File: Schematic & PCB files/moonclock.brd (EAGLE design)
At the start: 145 x 38.4 mm, 27 parts, among them U1 TCA9548APWR, U2 ESP32-S2-WROVER-I, U3 AMS1117-3.3, X2 BM04B-SRSS-TB

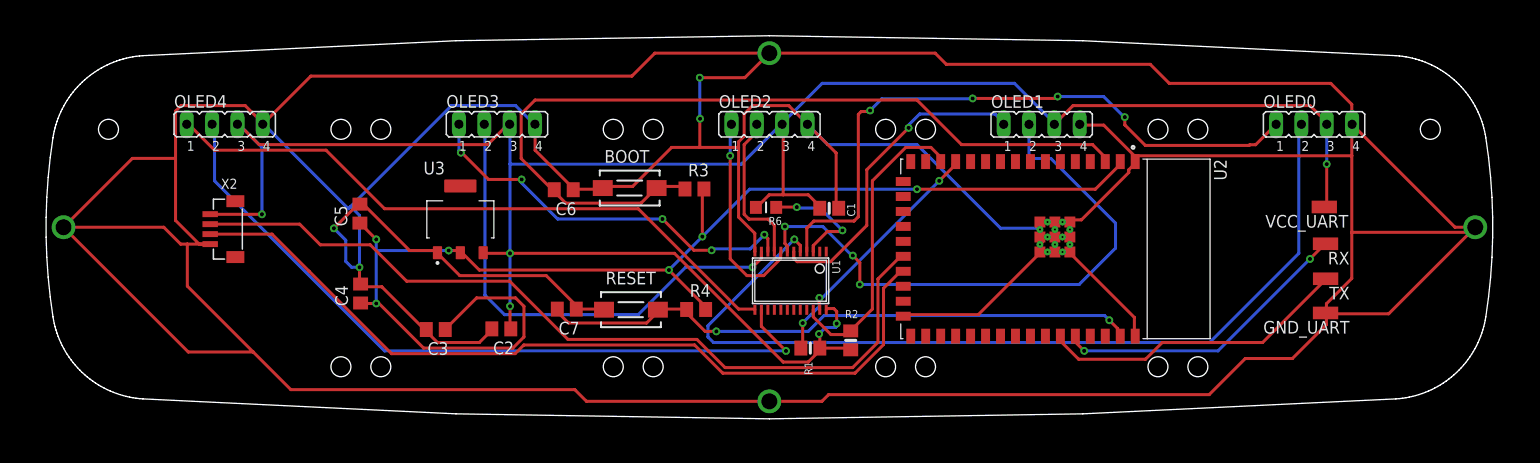
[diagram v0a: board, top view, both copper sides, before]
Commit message: Updated EAGLE files
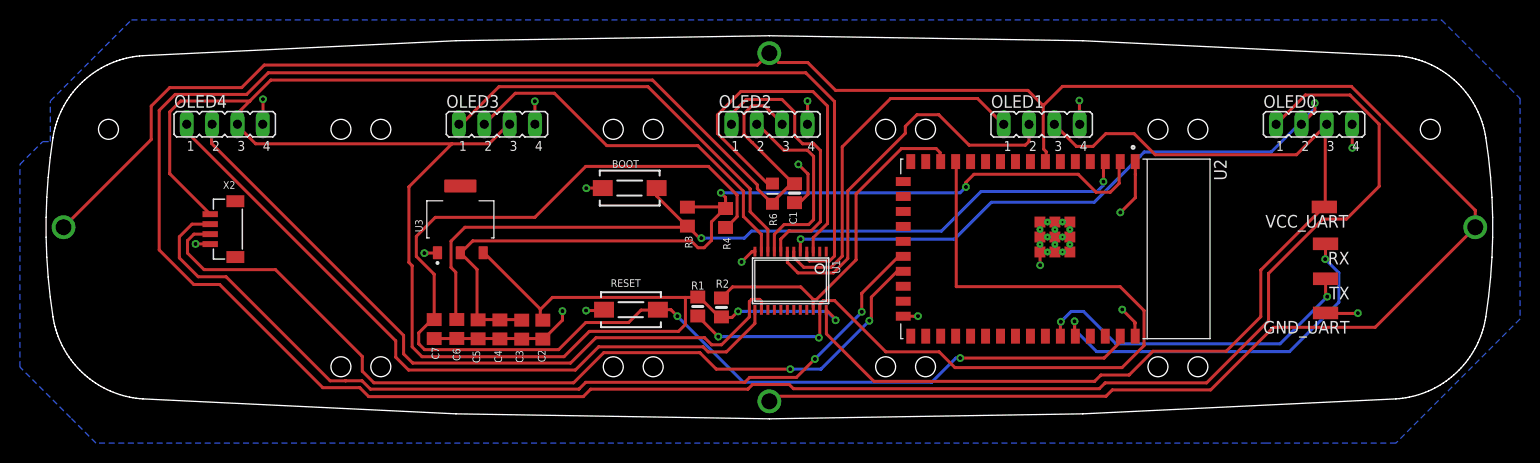
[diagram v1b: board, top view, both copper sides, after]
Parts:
- moved C6 17.6 mm to (43.3, 8.90), turned to 90 degrees
- moved C5 16.6 mm to (45.4, 8.87), turned to 270 degrees
- moved C4 14.4 mm to (47.6, 8.86), turned to 270 degrees
- moved C7 13.4 mm to (41.0, 8.89), turned to 90 degrees
- moved R2 13.4 mm to (69.8, 11.1)
- moved R1 12.0 mm to (67.4, 11.2), turned to 90 degrees
- moved R4 9.63 mm to (70.2, 20.0), turned to 90 degrees
- moved C3 8.62 mm to (49.8, 8.84), turned to 270 degrees
- moved C2 4.16 mm to (51.9, 8.84), turned to 270 degrees
- moved C1 3.79 mm to (77.1, 22.5), turned to 270 degrees
- moved R3 2.86 mm to (66.4, 20.2), turned to 90 degrees
- moved R6 1.52 mm to (74.9, 22.5), turned to 270 degrees
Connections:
- new net AGND: U2.7
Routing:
- net GND: track 673.1 -> 49.6 mm, vias 8 -> 17
- net AGND: track 0.00 -> 244.3 mm, vias 0 -> 4
- net 0SDA: track 64.3 -> 262.9 mm, vias 4 -> 0
- net VCC: track 225.2 -> 326.3 mm, vias 6 -> 2
- net N$10: track 60.8 -> 129.6 mm
- net INPUTSDA: track 26.6 -> 88.3 mm, vias 3 -> 2
- net N$7: track 130.9 -> 91.7 mm, vias 6 -> 2
- net 0SCL: track 91.1 -> 61.7 mm, vias 1 -> 2
- net RESET: track 11.8 -> 37.3 mm, vias 2 -> 0
- net 1SCL: track 58.1 -> 39.8 mm, vias 3 -> 0
- net 3SCL: track 48.7 -> 38.1 mm, vias 1 -> 0
- net N$6: track 30.5 -> 38.2 mm
- net 4SDA: track 64.7 -> 72.3 mm
- net D-: track 83.8 -> 90.4 mm, vias 0 -> 2
- net 2SDA: track 20.7 -> 27.1 mm, vias 1 -> 0
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- added copper zone on layer 16, net GND
